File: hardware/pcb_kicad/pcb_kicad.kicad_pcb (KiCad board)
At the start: 2 copper layers, 105.4 x 43.2 mm, 25 parts, among them J1 Screw_Terminal_01x02, J2 Screw_Terminal_01x02, J3 Screw_Terminal_01x02, J4 Screw_Terminal_01x02, J5 Screw_Terminal_01x02, J6 Conn_02x05_Top_Bottom, Q1 IRLB8721PBF, Q2 IRLB8721PBF, U1 LM7805_TO220

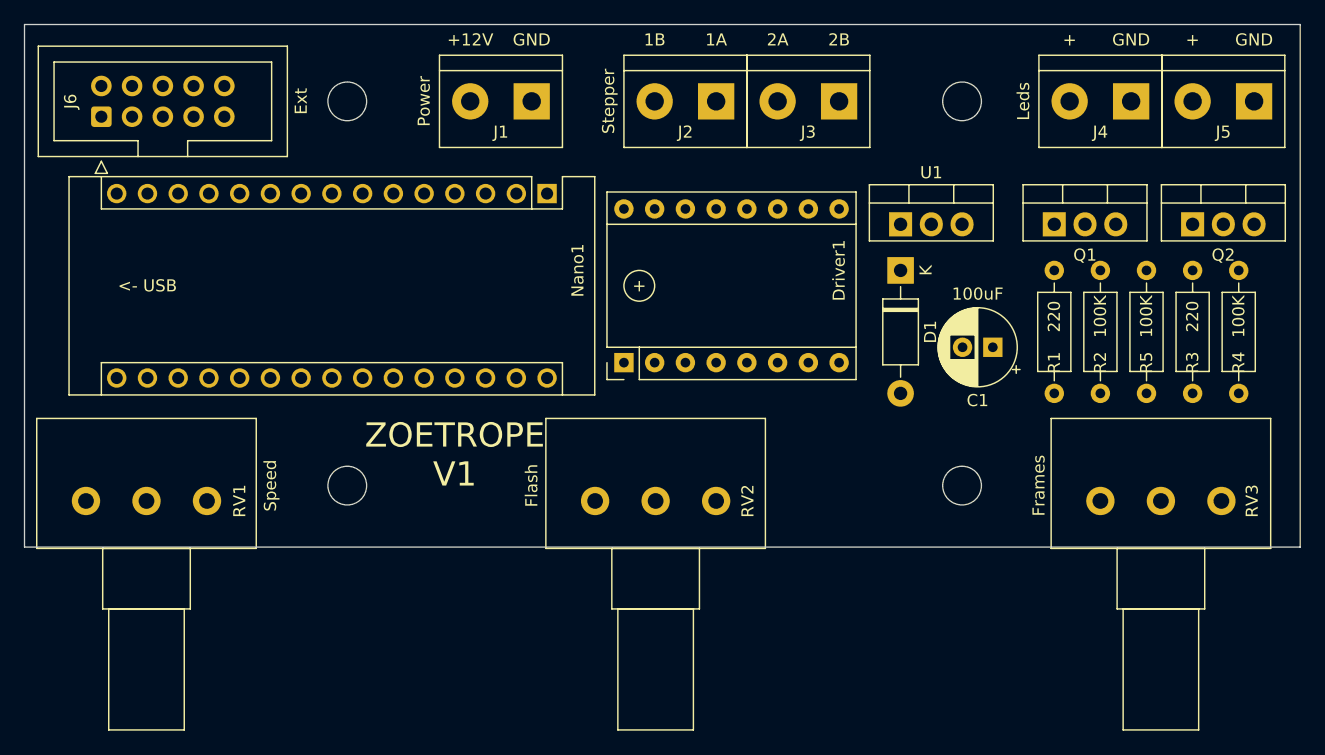
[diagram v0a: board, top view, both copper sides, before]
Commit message: v2 to be checked
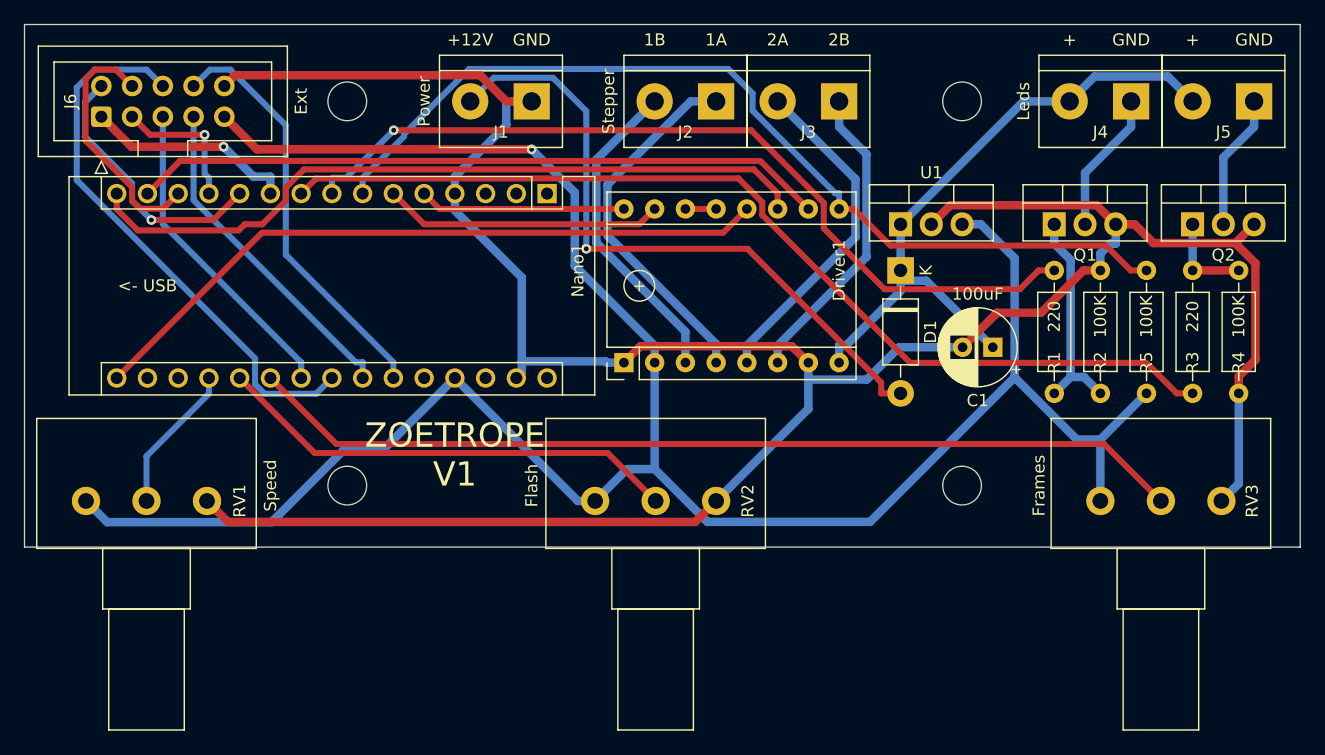
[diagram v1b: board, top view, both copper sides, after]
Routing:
- net GND: track 0.00 -> 223.7 mm
- net +5V: track 0.00 -> 186.6 mm, vias 0 -> 1
- net Net-(Nano1-Pad9): track 0.00 -> 82.2 mm
- net Net-(Driver1-Pad9): track 0.00 -> 78.4 mm
- net Net-(Nano1-Pad21): track 0.00 -> 77.8 mm
- net Net-(Nano1-Pad8): track 0.00 -> 69.9 mm, vias 0 -> 1
- net /MS2: track 0.00 -> 61.5 mm
- net /MS3: track 0.00 -> 57.9 mm
- net /MS1: track 0.00 -> 57.4 mm
- net Net-(D1-Pad2): track 0.00 -> 54.4 mm, vias 0 -> 1
- net +12V: track 0.00 -> 53.8 mm
- net Net-(J6-Pad6): track 0.00 -> 46.1 mm
- net Net-(Nano1-Pad20): track 0.00 -> 38.6 mm
- net Net-(J6-Pad8): track 0.00 -> 34.7 mm
- net Net-(Driver1-Pad4): track 0.00 -> 30.3 mm
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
